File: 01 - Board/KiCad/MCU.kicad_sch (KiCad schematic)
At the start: 2 parts, among them J3 Conn_ARM_SWD_TagConnect_TC2030, U3 STM32F030C8

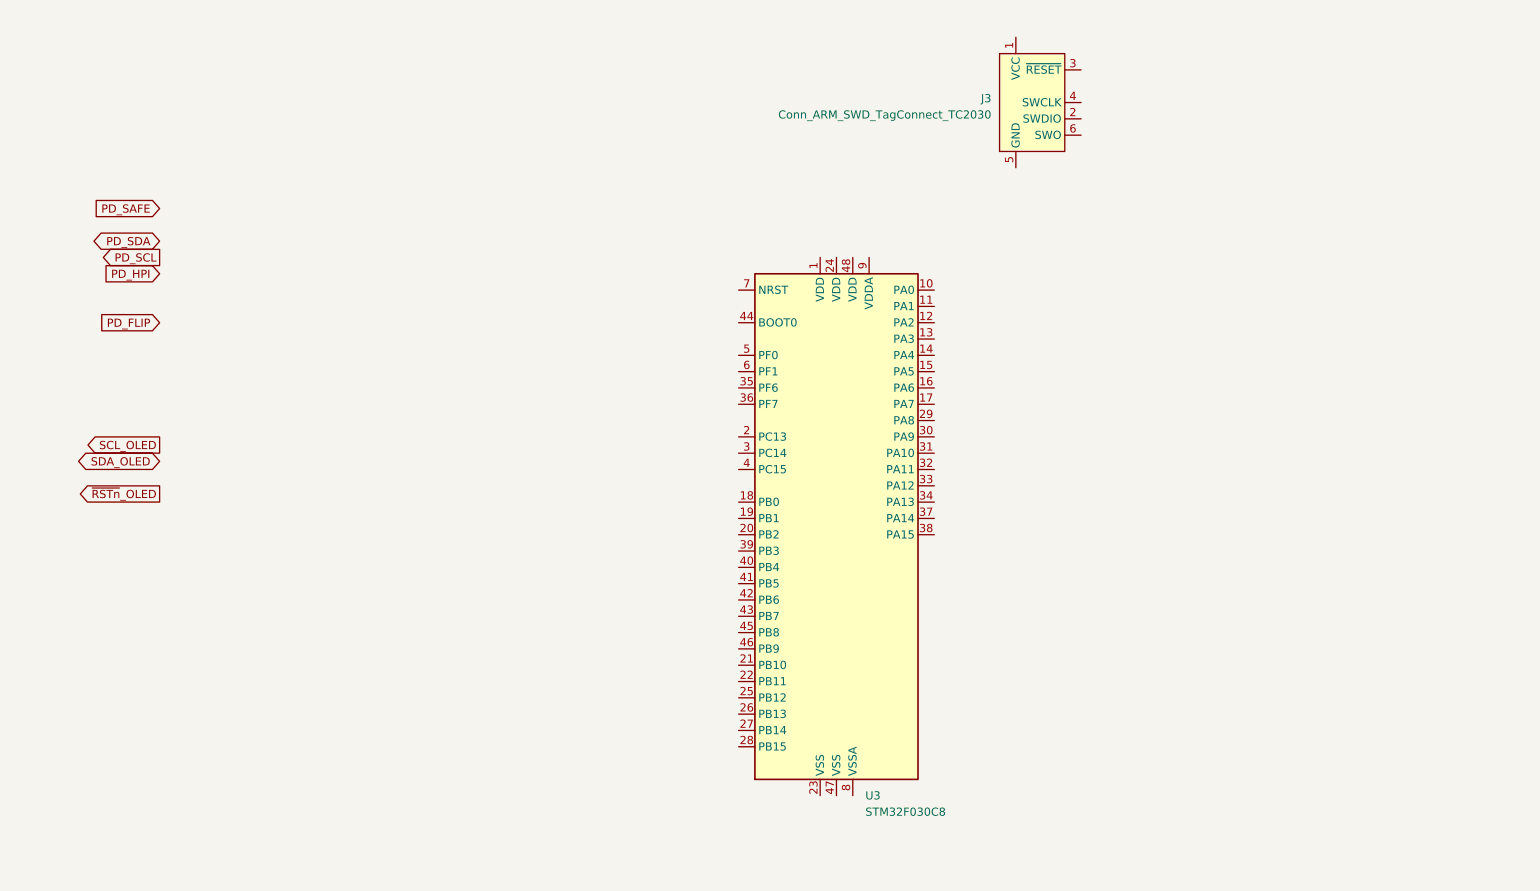
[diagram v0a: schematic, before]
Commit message: PCB order
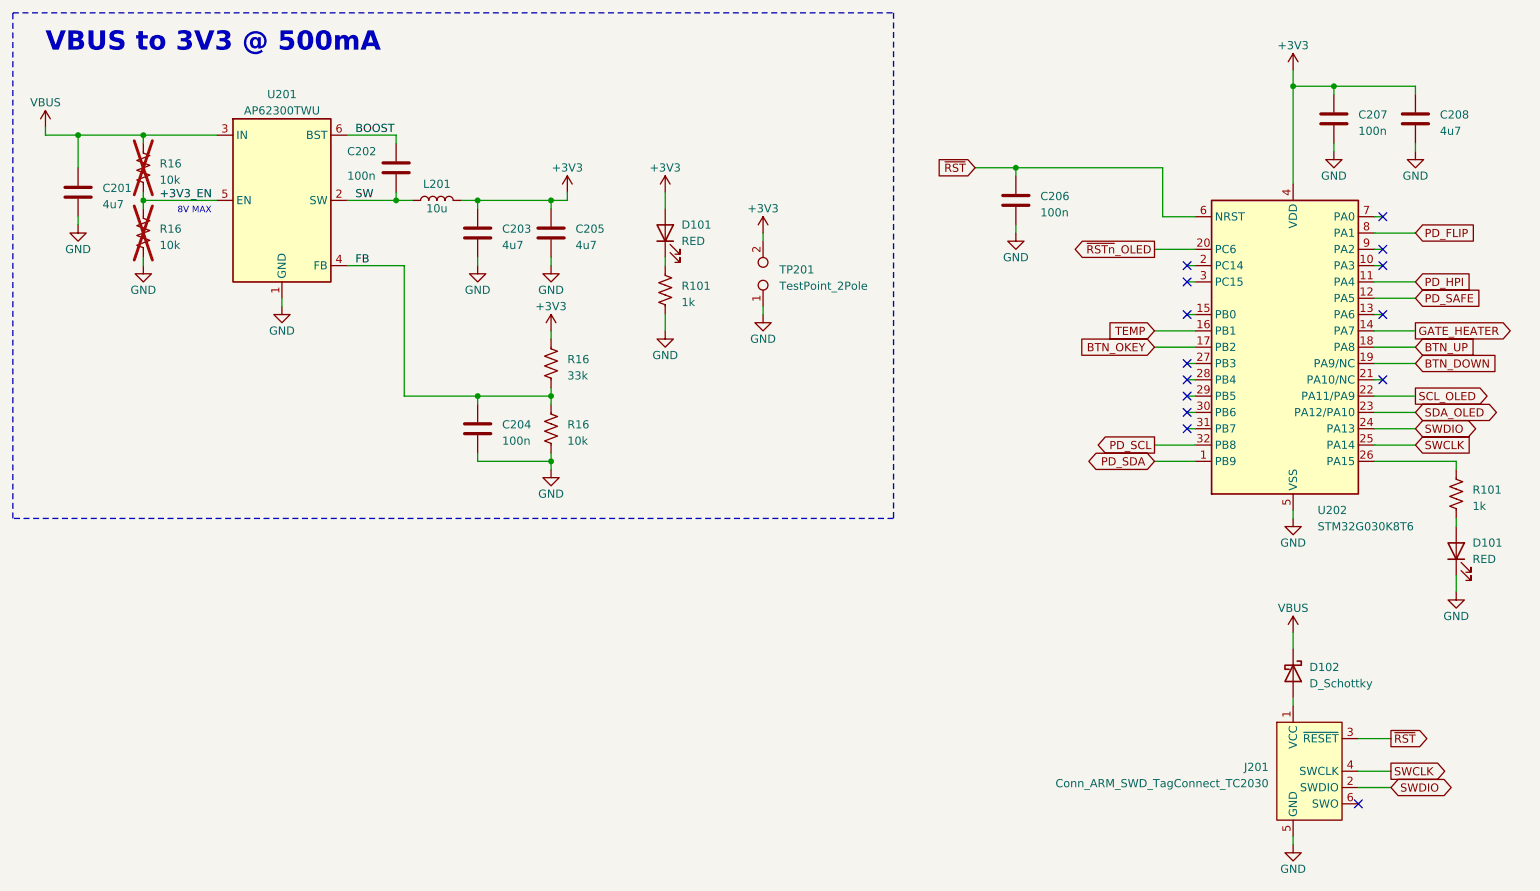
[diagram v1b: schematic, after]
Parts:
- removed U3: STM32F030C8, Package_QFP:LQFP-48_7x7mm_P0.5mm, symbol Symbols:STM32F030C8
- added C201, C203, C205, C208: 4u7, Capacitor_SMD:C_0805_2012Metric_Pad1.18x1.45mm_HandSolder, symbol Device:C
- added C202, C204, C206, C207: 100n, Capacitor_SMD:C_0603_1608Metric_Pad1.08x0.95mm_HandSolder, symbol Device:C
- added D101 (x2): RED, LED_SMD:LED_0603_1608Metric_Pad1.05x0.95mm_HandSolder, symbol Device:LED
- added D102: D_Schottky, Diode_SMD:D_SOD-323_HandSoldering, symbol Device:D_Schottky
- added L201: 10u, Footprints:L_4.2x4.4_H2, symbol Device:L
- added R101 (x2): 1k, Resistor_SMD:R_0603_1608Metric_Pad0.98x0.95mm_HandSolder, symbol Device:R_US
- added R16 (x3): 10k, Resistor_SMD:R_0603_1608Metric_Pad0.98x0.95mm_HandSolder, symbol Device:R_US
- added R16: 33k, Resistor_SMD:R_0603_1608Metric_Pad0.98x0.95mm_HandSolder, symbol Device:R_US
- added TP201: TestPoint_2Pole, Footprints:TestPoint_Pad_D1.0mm_DUAL, symbol Connector:TestPoint_2Pole
- added U201: AP62300TWU, Package_TO_SOT_SMD:TSOT-23-6, symbol Symbols:AP62300TWU
- added U202: STM32G030K8T6, Package_QFP:LQFP-32_7x7mm_P0.8mm, symbol MCU_ST_STM32G0:STM32G030K8Tx
- renumbered J3 to J201
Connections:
- net PD_FLIP: now also U202.8 (PA1)
- net PD_HPI: now also U202.11 (PA4)
- net PD_SAFE: now also U202.12 (PA5)
- net PD_SCL: now also U202.32 (PB8)
- net PD_SDA: now also U202.1 (PB9)
- net SCL_OLED: now also U202.22 (PA11/PA9)
- net SDA_OLED: now also U202.23 (PA12/PA10)
- net ~{RSTn}_OLED: now also U202.20 (PC6)
- net at J201.1 (VCC): now also D102.2 (A)
- net SWDIO: now reaches J201.2 (SWDIO)
- net SWDIO: now also U202.24 (PA13)
- net ~{RST}: now reaches J201.3 (~{RESET})
- net ~{RST}: now also C206.1, U202.6 (NRST)
- net SWCLK: now reaches J201.4 (SWCLK)
- net SWCLK: now also U202.25 (PA14)
- net GND: now reaches J201.5 (GND)
- net GND: now also C201.2, C203.2, C204.2, C205.2, C206.2, C207.2, C208.2, D101.1 (K), R101.2, R16.2, R16.2, TP201.1, U201.1 (GND), U202.5 (VSS)
- new net: D101.1 (K), R101.1
- new net: R101.1, U202.26 (PA15)
- new net: D101.2 (A), R101.2
- new net +3V3: C203.1, C205.1, C207.1, C208.1, D101.2 (A), L201.2, R16.1, TP201.2, U202.4 (VDD)
- new net +3V3_EN: R16.1, R16.2, U201.5 (EN)
- new net BOOST: C202.1, U201.6 (BST)
- new net BTN_DOWN: U202.19 (PA9/NC)
- new net BTN_OKEY: U202.17 (PB2)
- new net BTN_UP: U202.18 (PA8)
- new net FB: C204.1, R16.1, R16.2, U201.4 (FB)
- new net GATE_HEATER: U202.14 (PA7)
- new net SW: C202.2, L201.1, U201.2 (SW)
- new net TEMP: U202.16 (PB1)
- new net VBUS: C201.1, D102.1 (K), R16.1, U201.3 (IN)
- no-connect marks 0 -> 14
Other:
- note added: "8V MAX"
- note added: "VBUS to 3V3 @ 500mA"
- moved on the sheet: J201
